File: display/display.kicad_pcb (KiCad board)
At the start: 2 copper layers, 19 parts, among them J1 DIN41612_03x32_ABC

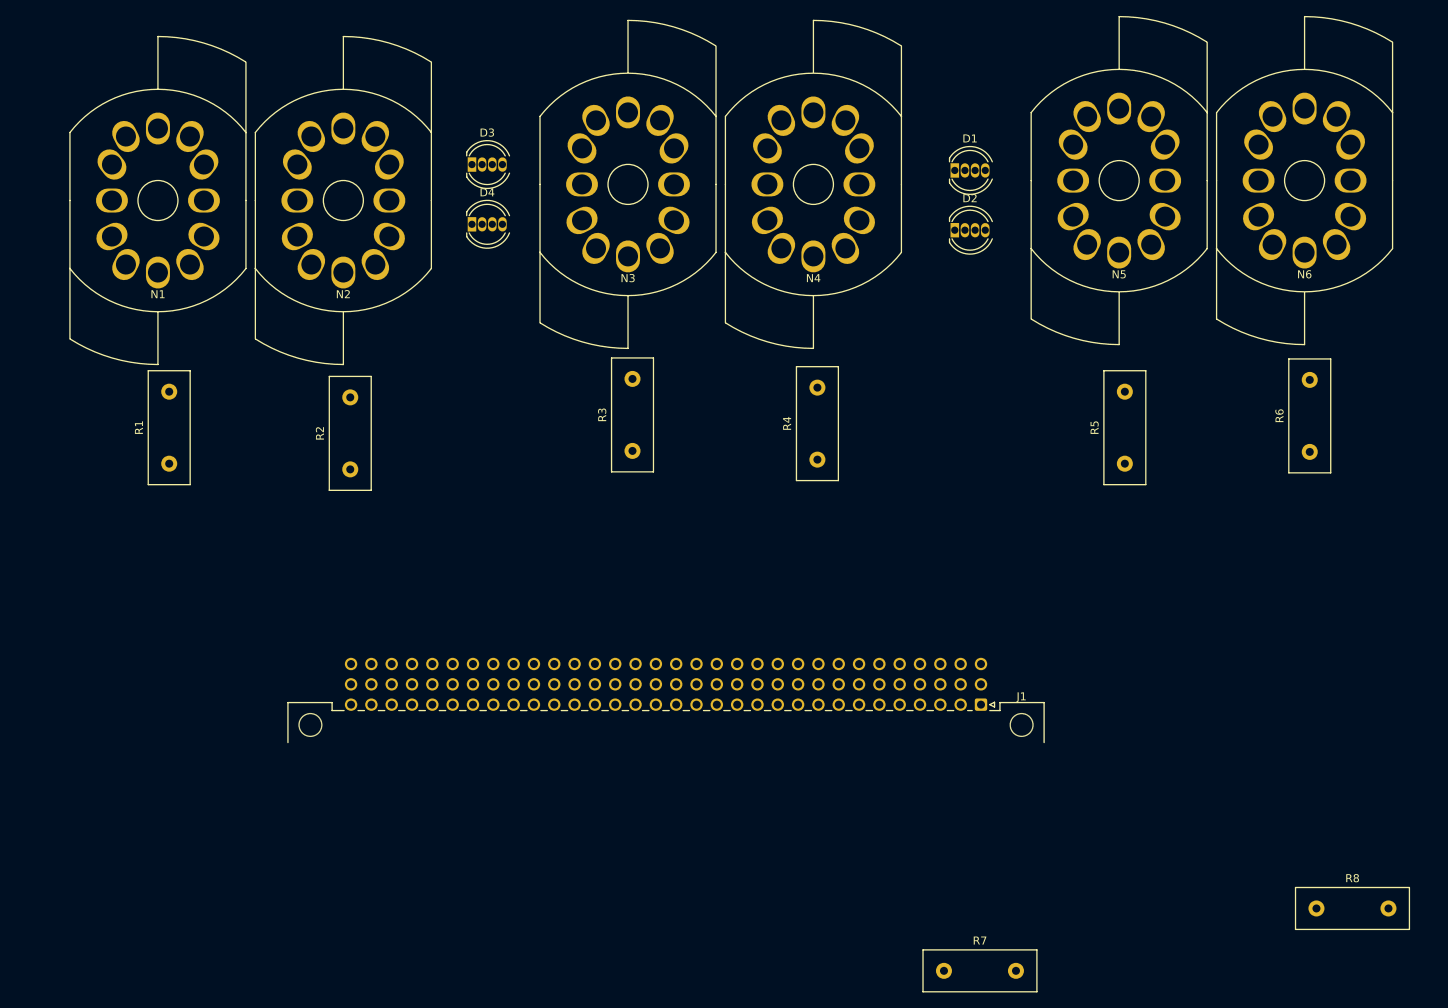
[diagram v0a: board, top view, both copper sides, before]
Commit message: Layout is ongoing
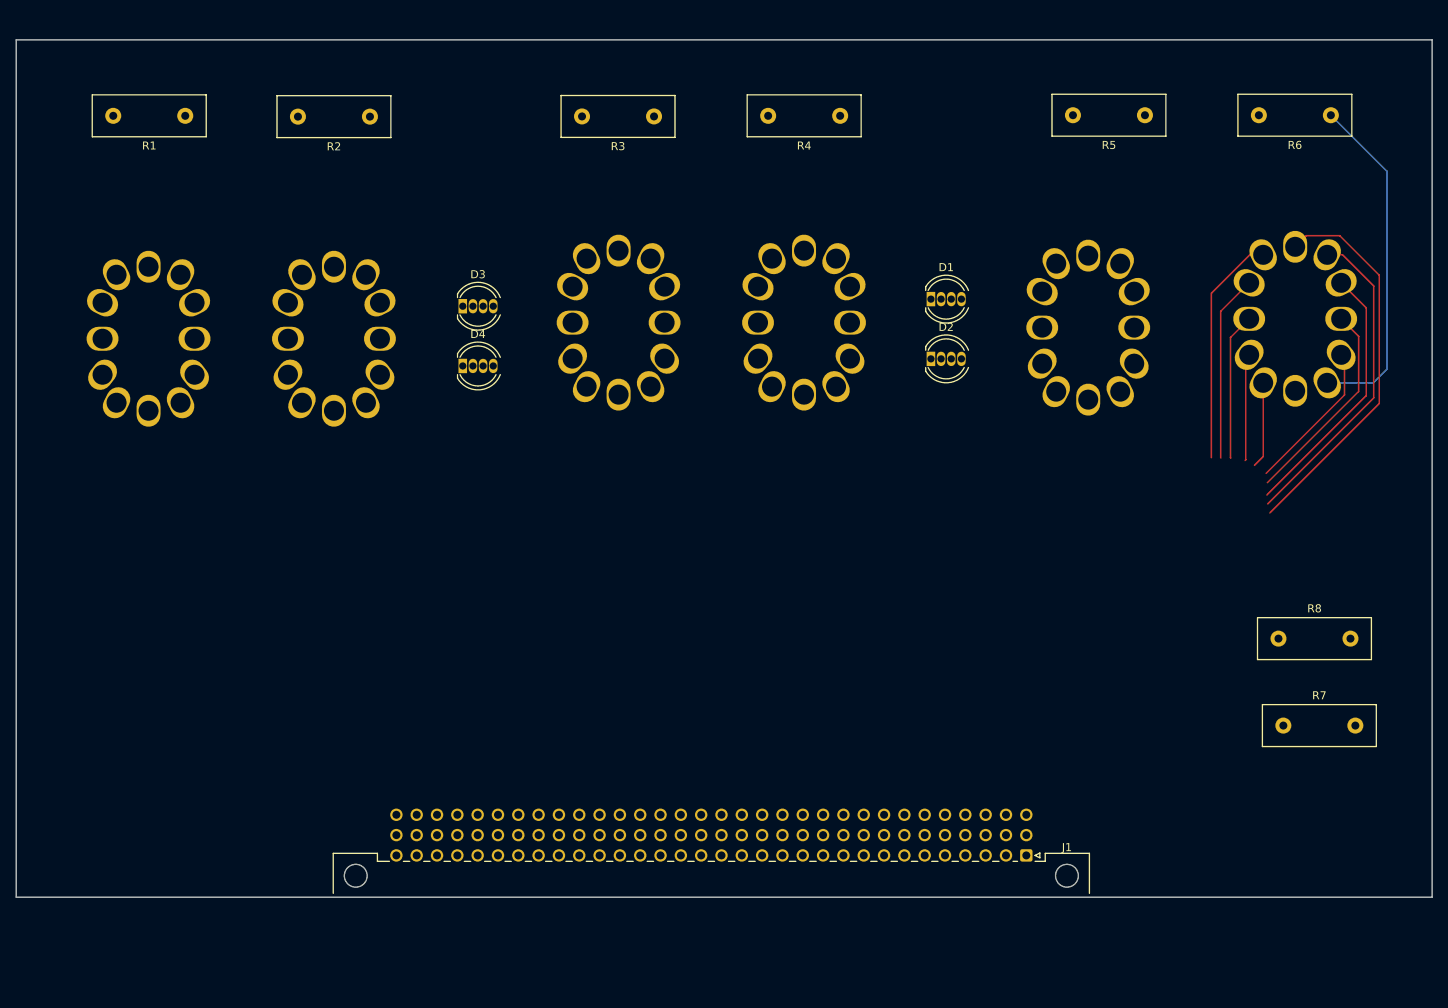
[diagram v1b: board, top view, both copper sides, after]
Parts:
- N1, N2, N3, N4, N5, N6: moved to B.Cu
- moved R7 52.3 mm to (212.6, 105.8)
- moved R2 44.2 mm to (98.4, 29.7), turned to 180 degrees
- moved R5 43.6 mm to (195.3, 29.5), turned to 180 degrees
- moved R1 43.5 mm to (75.3, 29.6), turned to 180 degrees
- moved R4 43.1 mm to (157.2, 29.6), turned to 180 degrees
- moved R6 42.2 mm to (218.5, 29.5), turned to 180 degrees
- moved R3 41.9 mm to (133.9, 29.6), turned to 180 degrees
- moved R8 34.1 mm to (212.0, 94.9)
- moved J1 19.7 mm to (180.4, 122.0)
- moved N5 18.8 mm to (188.2, 56.0)
- moved D3 17.7 mm to (110.0, 53.4)
- moved D4 17.7 mm to (110.0, 60.8)
- moved N3 17.3 mm to (129.5, 55.4)
- moved N4 17.3 mm to (152.7, 55.4)
- moved N6 17.3 mm to (214.1, 54.9)
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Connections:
- J1 pad c1: /T4-0 -> /T6-6
- J1 pad c10: /T4-9 -> /T6-5
- J1 pad c11: /T5-0 -> /T5-9
- J1 pad c12: /T5-1 -> /T5-8
- J1 pad c13: /T5-2 -> /T5-7
- J1 pad c14: /T5-3 -> /T5-6
- J1 pad c15: /T5-4 -> /T5-5
- J1 pad c16: /T5-5 -> /T5-4
- J1 pad c17: /T5-6 -> /T5-3
- J1 pad c18: /T5-7 -> /T5-2
- J1 pad c19: /T5-8 -> /T5-1
- J1 pad c2: /T4-1 -> /T6-7
- J1 pad c20: /T5-9 -> /T5-0
- J1 pad c21: /T6-0 -> /T4-9
- J1 pad c22: /T6-1 -> /T4-8
- J1 pad c23: /T6-2 -> /T4-7
- J1 pad c24: /T6-3 -> /T4-6
- J1 pad c25: /T6-4 -> /T4-5
- J1 pad c26: /T6-5 -> /T4-4
- J1 pad c27: /T6-6 -> /T4-3
- J1 pad c28: /T6-7 -> /T4-2
- J1 pad c29: /T6-8 -> /T4-1
- J1 pad c3: /T4-2 -> /T6-8
- J1 pad c30: /T6-9 -> /T4-0
- J1 pad c4: /T4-3 -> /T6-9
- J1 pad c5: /T4-4 -> /T6-0
- J1 pad c6: /T4-5 -> /T6-1
- J1 pad c7: /T4-6 -> /T6-2
- J1 pad c8: /T4-7 -> /T6-3
- J1 pad c9: /T4-8 -> /T6-4
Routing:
- net /T6-6: track 0.00 -> 48.5 mm
- net Net-(N6-A): track 0.00 -> 42.9 mm
- net /T6-7: track 0.00 -> 42.9 mm
- net /T6-8: track 0.00 -> 33.0 mm
- net /T6-5: track 0.00 -> 29.0 mm
- net /T6-9: track 0.00 -> 26.1 mm
- net /T6-4: track 0.00 -> 23.4 mm
- net /T6-0: track 0.00 -> 19.7 mm
- net /T6-3: track 0.00 -> 18.4 mm
- net /T6-2: track 0.00 -> 13.4 mm
- net /T6-1: track 0.00 -> 10.8 mm
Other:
- board outline added: 177 x 107.2 mm
